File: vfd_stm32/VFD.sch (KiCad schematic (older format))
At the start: 25 parts, among them U1 DC201LA, U10 74HC595, U11 74HC595, U12 74HC595, U13 74HC595, U14 74HC595, U15 74HC595, U16 74HC595, U17 74HC595, U2 ULN2003, U3 ULN2003, U4 ULN2003, U5 ULN2003, U6 ULN2003, U7 ULN2003, U8 ULN2003, U9 ULN2003

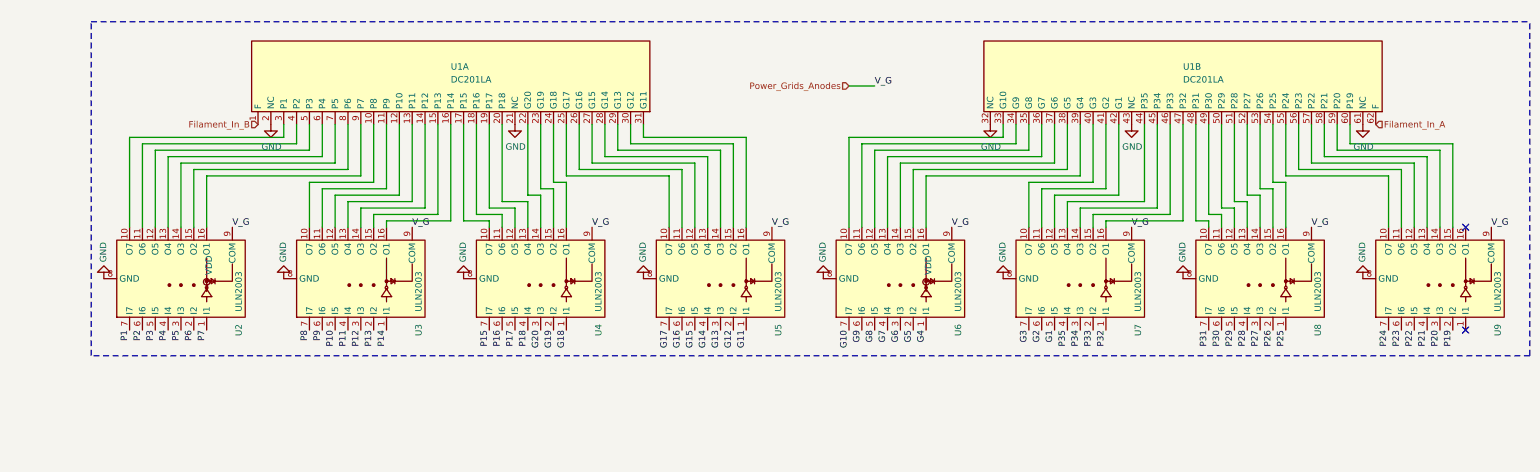
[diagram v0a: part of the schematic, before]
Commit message: continue circuitry
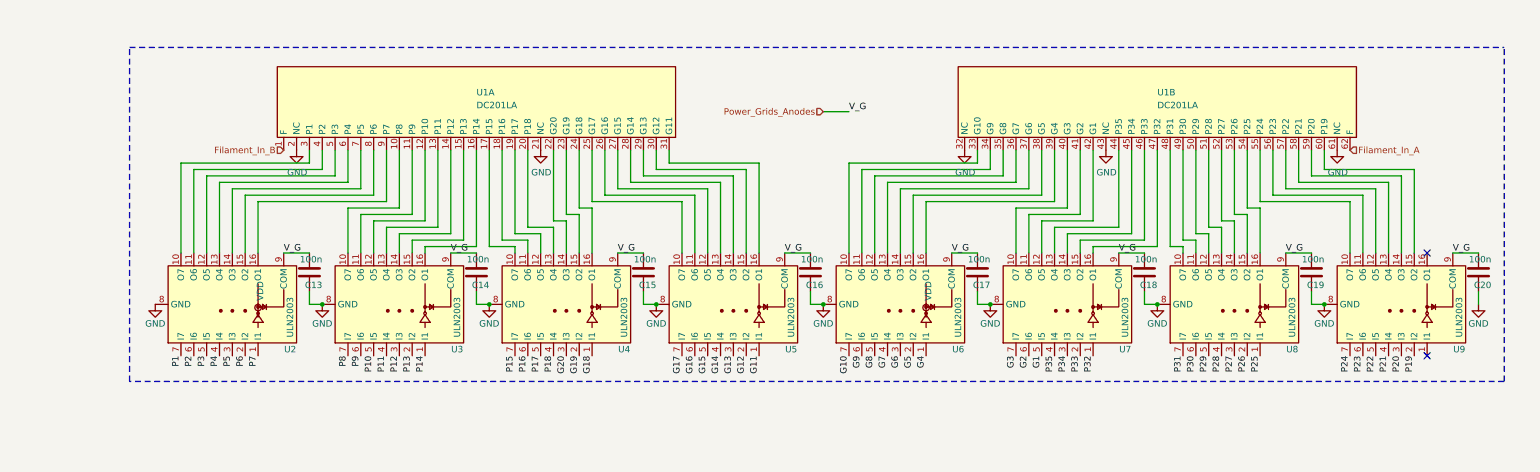
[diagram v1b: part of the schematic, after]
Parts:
- added C13, C14, C15, C16, C17, C18, C19, C20: 100n, Capacitor_SMD:C_0805_2012Metric_Pad1.15x1.40mm_HandSolder, symbol Device:C
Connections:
- wire segments 193 -> 216
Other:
- moved on the sheet: U1A, U1B, U2, U3, U4, U5, U6, U7, U8, U9

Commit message: todo
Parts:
- added J1, J2: Conn_01x04, symbol Connector_Generic:Conn_01x05
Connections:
- net labels added: RCLK1, RCLK2, SPI_Grids_Anodes_1_out, SPI_Grids_Anodes_2, SRCLK1, SRCLK2
- wire segments 216 -> 211
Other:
- moved on the sheet: C10, C11, C13, C14, C15, C16, C17, C18, C19, C20, C4, C5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
